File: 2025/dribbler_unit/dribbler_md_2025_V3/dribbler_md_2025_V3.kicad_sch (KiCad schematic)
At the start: 113 parts, among them J2 Conn_01x04_Pin, J3 Conn_01x02_Pin, J4 Conn_01x07_Pin, J5 Conn_01x03_Pin, J6 Conn_01x02_Pin, J7 Conn_01x02_Pin, J8 Conn_01x02_Socket, SW2 SW_MEC_5E, SW4 SW_MEC_5E, U1 MAX3051, U2 STS8DN3LLH5, U3 STS8DN3LLH5, U4 DRV8701, U5 STM32F446RETx, Y1 Crystal_GND2

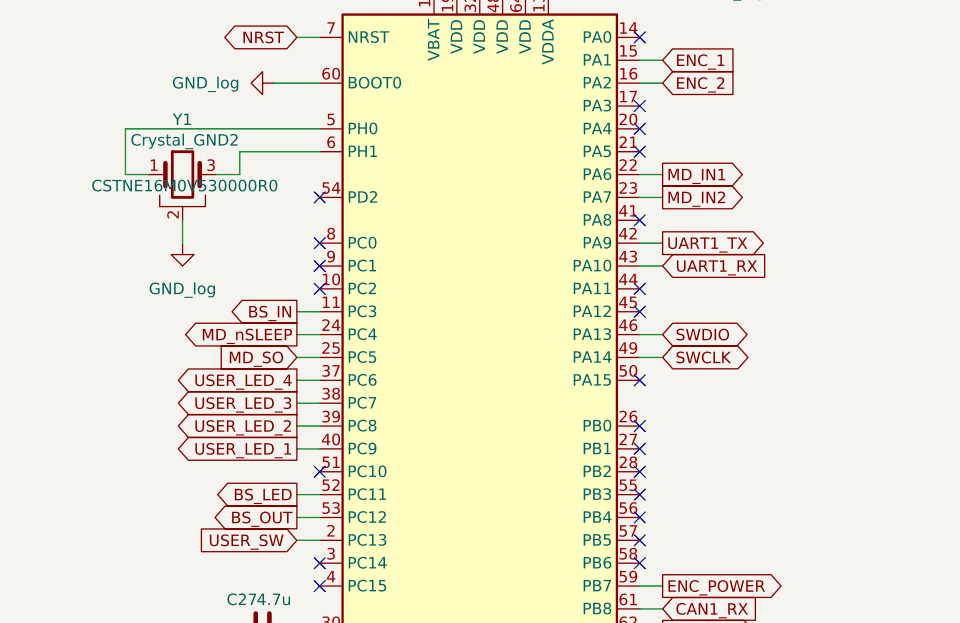
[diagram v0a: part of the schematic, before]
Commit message: ピン配置変更
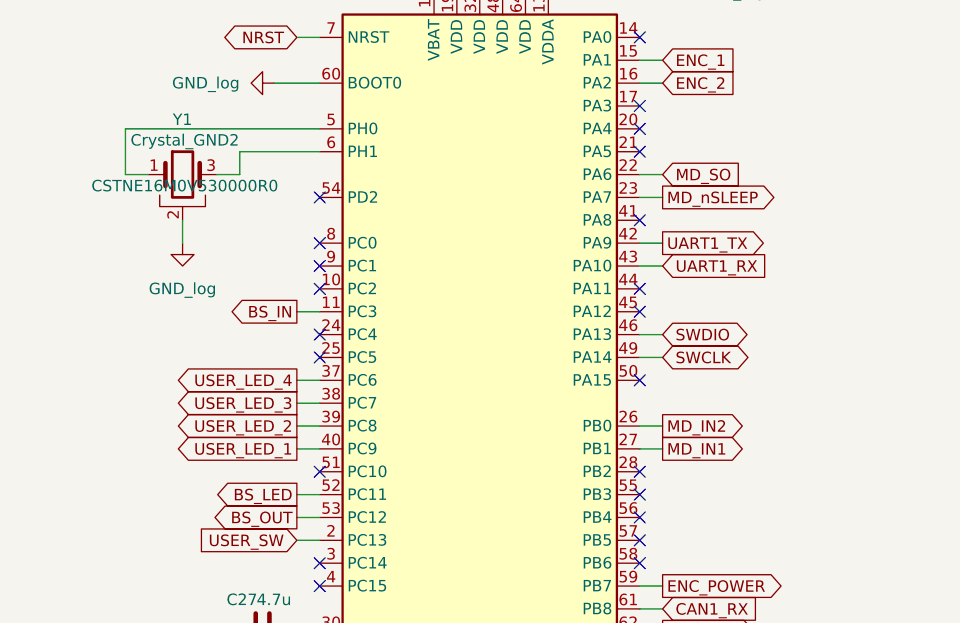
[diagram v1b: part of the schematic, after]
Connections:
- net MD_IN1: now also U5.27 (PB1); no longer U5.22 (PA6)
- net MD_IN2: now also U5.26 (PB0); no longer U5.23 (PA7)
- net MD_SO: now also U5.22 (PA6); no longer U5.25 (PC5)
- net MD_nSLEEP: now also U5.23 (PA7); no longer U5.24 (PC4)
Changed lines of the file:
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@@
 	)
 	(no_connect
-		(at 241.3 102.87)
+		(at 241.3 130.81)
 	)
 	(no_connect
-		(at 241.3 130.81)
+		(at 205.74 95.25)
 	)
 	(no_connect
@@
 	)
 	(no_connect
-		(at 241.3 105.41)
-	)
-	(no_connect
 		(at 241.3 115.57)
 	)
@@
 	)
 	(no_connect
+		(at 205.74 92.71)
+	)
+	(no_connect
 		(at 205.74 87.63)
 	)
@@
 	(wire
 		(pts
-			(xy 203.2 95.25) (xy 205.74 95.25)
-		)
-		(stroke
-			(width 0)
-			(type default)
-		)
-	)
-	(wire
-		(pts
 			(xy 36.83 62.23) (xy 41.91 62.23)
 		)
@@
 	(wire
 		(pts
+			(xy 241.3 105.41) (xy 243.84 105.41)
+		)
+		(stroke
+			(width 0)
+			(type default)
+		)
+	)
+	(wire
+		(pts
 			(xy 110.49 57.15) (xy 138.43 57.15)
 		)
@@
 	(wire
 		(pts
+			(xy 241.3 74.93) (xy 243.84 74.93)
+		)
+		(stroke
+			(width 0)
+			(type default)
+		)
+	)
+	(wire
+		(pts
 			(xy 303.53 158.75) (xy 303.53 161.29)
 		)
@@
 	(wire
 		(pts
-			(xy 241.3 77.47) (xy 243.84 77.47)
-		)
-		(stroke
-			(width 0)
-			(type default)
-		)
-	)
-	(wire
-		(pts
 			(xy 129.54 194.31) (xy 129.54 191.77)
 		)
@@
 	(wire
 		(pts
+			(xy 241.3 102.87) (xy 243.84 102.87)
+		)
+		(stroke
+			(width 0)
+			(type default)
+		)
+	)
+	(wire
+		(pts
 			(xy 218.44 52.07) (xy 220.98 52.07)
 		)
@@
 	(wire
 		(pts
-			(xy 203.2 92.71) (xy 205.74 92.71)
-		)
-		(stroke
-			(width 0)
-			(type default)
-		)
-	)
-	(wire
-		(pts
 			(xy 31.75 74.93) (xy 36.83 74.93)
 		)
@@
 	(wire
 		(pts
+			(xy 241.3 77.47) (xy 243.84 77.47)
+		)
+		(stroke
+			(width 0)
+			(type default)
+		)
+	)
+	(wire
+		(pts
 			(xy 15.24 36.83) (xy 15.24 38.1)
 		)
@@
 	(wire
 		(pts
-			(xy 241.3 74.93) (xy 243.84 74.93)
-		)
-		(stroke
-			(width 0)
-			(type default)
-		)
-	)
-	(wire
-		(pts
 			(xy 302.26 69.85) (xy 304.8 69.85)
 		)
@@
 	(global_label "MD_SO"
 		(shape input)
-		(at 203.2 95.25 180)
+		(at 243.84 74.93 0)
 		(fields_autoplaced yes)
 		(effects
@@
 				(size 1.27 1.27)
 			)
-			(justify right)
+			(justify left)
 		)
 		(property "Intersheetrefs" "${INTERSHEET_REFS}"
-			(at 193.9858 95.25 0)
+			(at 253.0542 74.93 0)
 			(effects
 				(font
 					(size 1.27 1.27)
 				)
-				(justify right)
+				(justify left)
 				(hide yes)
 			)
@@
 	(global_label "MD_nSLEEP"
 		(shape output)
-		(at 203.2 92.71 180)
+		(at 243.84 77.47 0)
 		(fields_autoplaced yes)
 		(effects
@@
 				(size 1.27 1.27)
 			)
-			(justify right)
+			(justify left)
 		)
 		(property "Intersheetrefs" "${INTERSHEET_REFS}"
-			(at 189.5712 92.71 0)
+			(at 257.4688 77.47 0)
 			(effects
 				(font
 					(size 1.27 1.27)
 				)
-				(justify right)
+				(justify left)
 				(hide yes)
 			)
@@
 	(global_label "MD_IN2"
 		(shape output)
-		(at 243.84 77.47 0)
+		(at 243.84 102.87 0)
 		(fields_autoplaced yes)
 		(effects
@@
 		)
 		(property "Intersheetrefs" "${INTERSHEET_REFS}"
-			(at 253.659 77.47 0)
+			(at 253.659 102.87 0)
 			(effects
 				(font
@@
 	(global_label "MD_IN1"
 		(shape output)
-		(at 243.84 74.93 0)
+		(at 243.84 105.41 0)
 		(fields_autoplaced yes)
 		(effects
@@
 		)
 		(property "Intersheetrefs" "${INTERSHEET_REFS}"
-			(at 253.659 74.93 0)
+			(at 253.659 105.41 0)
 			(effects
 				(font
